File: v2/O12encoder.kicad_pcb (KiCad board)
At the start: 2 copper layers, 14 x 14 mm, 17 parts, among them J1 Conn_01x06_Pin, J2 Conn_01x06_Pin, J4 Conn_01x06_Pin, J5 JST_SM02B-SRSS-TB(LF)(SN), J6 Conn_01x06_Pin, J7 Conn_01x06_Pin, J8 Conn_01x06_Pin, U1 MA702GQ-P, U2 STM32L011F4Ux, U3 THVD1420DRLR

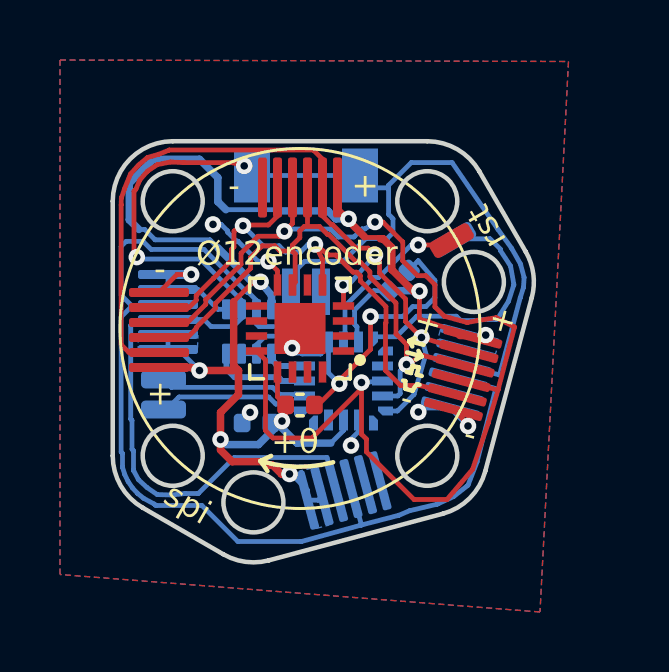
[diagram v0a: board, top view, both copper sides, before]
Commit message: readme, gen pdf
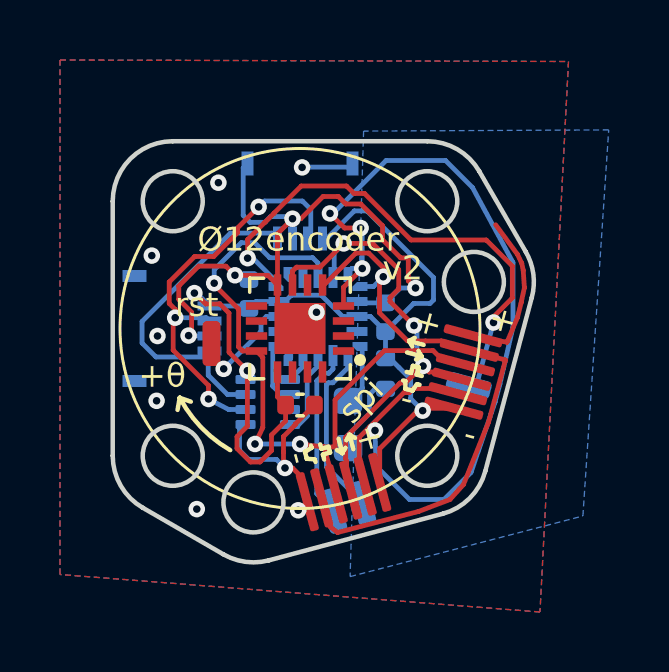
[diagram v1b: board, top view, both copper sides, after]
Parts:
- removed J5: JST_SM02B-SRSS-TB(LF)(SN), O32controller:JST_SM02B-SRSS-TB(LF)(SN)
- removed J6, J7, J8: Conn_01x06_Pin, O32controller:FFC_0.5mm_6p
- added D1: LED_Small, LED_SMD:LED_0603_1608Metric, B.Cu at (51.6, 53.2)
- added J3: Conn_01x04, O12encoder:TE_2328702-4, B.Cu at (50.0, 45.5)
- added R1: R_Small_US, Resistor_SMD:R_0402_1005Metric, B.Cu at (52.9, 51.5)
- J1, J2: footprint O32controller:FFC_0.5mm_6p -> O12encoder:FFC_0.5mm_6p
- J4: value Conn_01x06_Pin -> Conn_01x04; footprint O32controller:FFC_0.5mm_6p -> O12encoder:TE_2328702-4; moved to B.Cu
- TP1, TP2, TP3, TP4: footprint O32controller:TestPoint_Pad_Rect -> O12encoder:TestPoint_Pad_Rect
- U1: footprint O32controller:MA702GQ-P -> O12encoder:MA702GQ-P
- U3: footprint O32controller:THVD1420DRLR_SOT-585 -> O12encoder:THVD1420DRLR_SOT-585
- moved J4 10.00 mm to (45.5, 50.0), turned to 90 degrees
- moved TP1 8.70 mm to (47.0, 50.5), turned to 180 degrees
- moved J2 8.59 mm to (55.8, 50.2), turned to -15 degrees
- moved J1 8.55 mm to (50.2, 55.8), turned to 105 degrees
- moved TP2 7.34 mm to (52.1, 55.8), turned to 15 degrees
- moved TP3 7.17 mm to (51.1, 56.1), turned to 15 degrees
- moved C2 5.56 mm to (52.9, 49.6), turned to 90 degrees
- moved C3 5.02 mm to (48.3, 48.9), turned to 90 degrees
- moved TP4 4.90 mm to (55.6, 51.9), turned to -105 degrees
- moved U3 2.43 mm to (48.9, 52.5), turned to 180 degrees
- moved U2 2.31 mm to (50.6, 49.6), turned to 0 degrees
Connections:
- J4 pad 1: GND -> +3.3V
- J4 pad 2: /~{MAG2_CS} -> /RS485_A
- J4 pad 3: /SPI_SCLK -> GND
- J4 pad 4: /SPI_MISO -> /RS485_B
- U2 pad 11: unconnected-(U2-PB1-Pad11) -> /~{MAG2_CS}
- U2 pad 15: unconnected-(U2-PA10-Pad15) -> Net-(D1-K)
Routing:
- net /RS485_A: track 50.9 -> 14.1 mm, vias 2 -> 3
- net /RS485_B: track 37.4 -> 11.4 mm
- net +3.3V: track 50.7 -> 33.6 mm, vias 8 -> 3
- net /SPI_SCLK: track 38.0 -> 21.4 mm
- net GND: track 23.9 -> 38.0 mm, vias 10 -> 13
- net /ADC_IN0/WKUP: track 8.72 -> 17.5 mm, vias 0 -> 2
- net /SPI_MISO: track 19.2 -> 15.2 mm, vias 1 -> 3
- net Net-(D1-A): track 0.00 -> 2.54 mm
- net Net-(D1-K): track 0.00 -> 2.06 mm
- net /NRST: track 5.67 -> 3.65 mm
- net /SPI_MOSI: track 28.5 -> 29.9 mm, vias 3 -> 4
- net /SWCLK: track 4.86 -> 5.72 mm
- net /SWDIO: track 4.86 -> 5.63 mm
- net /~{MAG2_CS}: track 18.6 -> 18.7 mm, vias 2 -> 1
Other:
- board text added: "+ a"
- board text added: "- b"
- board text added: "rs485+"
- board text added: "v2"
- board text removed: "a"
- board text removed: "b"
- board text removed: "rs485"
